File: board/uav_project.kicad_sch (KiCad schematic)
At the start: 17 parts, among them J2 Conn_01x08_Pin

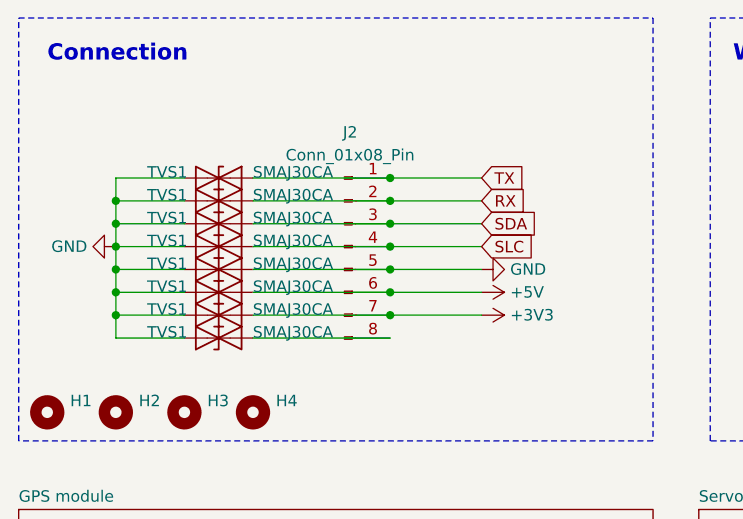
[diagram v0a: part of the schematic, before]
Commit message: More work on PCB design
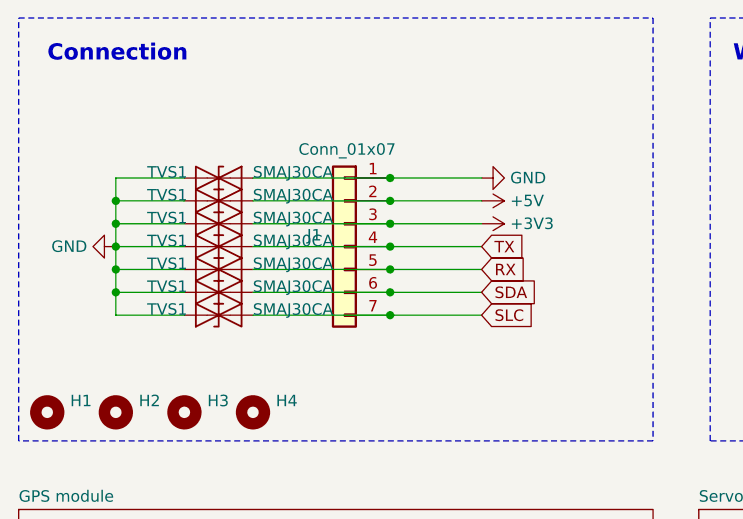
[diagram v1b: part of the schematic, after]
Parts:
- removed J2: Conn_01x08_Pin, Connector_PinHeader_1.00mm:PinHeader_1x08_P1.00mm_Vertical, symbol Connector:Conn_01x08_Pin
- removed TVS1: SMAJ30CA, Diode_SMD:D_SMA, symbol Diode:SMAJ30CA
- added J1: Conn_01x07, Connector_PinHeader_1.00mm:PinHeader_1x07_P1.00mm_Vertical, symbol Connector_Generic:Conn_01x07
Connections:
- net +3V3: now also TVS1.1 (A1), J1.3 (Pin_3); no longer TVS1.1 (A1)
- net +5V: now also TVS1.1 (A1), J1.2 (Pin_2); no longer TVS1.1 (A1)
- net GND: now also TVS1.1 (A1), J1.1 (Pin_1); no longer TVS1.1 (A1)
- net RX: now also TVS1.1 (A1), J1.5 (Pin_5); no longer TVS1.1 (A1)
- net SDA: now also TVS1.1 (A1), J1.6 (Pin_6); no longer TVS1.1 (A1)
- net SLC: now also TVS1.1 (A1), J1.7 (Pin_7); no longer TVS1.1 (A1)
- net TX: now also TVS1.1 (A1), J1.4 (Pin_4); no longer TVS1.1 (A1)
